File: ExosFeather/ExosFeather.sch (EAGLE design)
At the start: 3 parts, among them J1 CONN_3X1_JST_PA

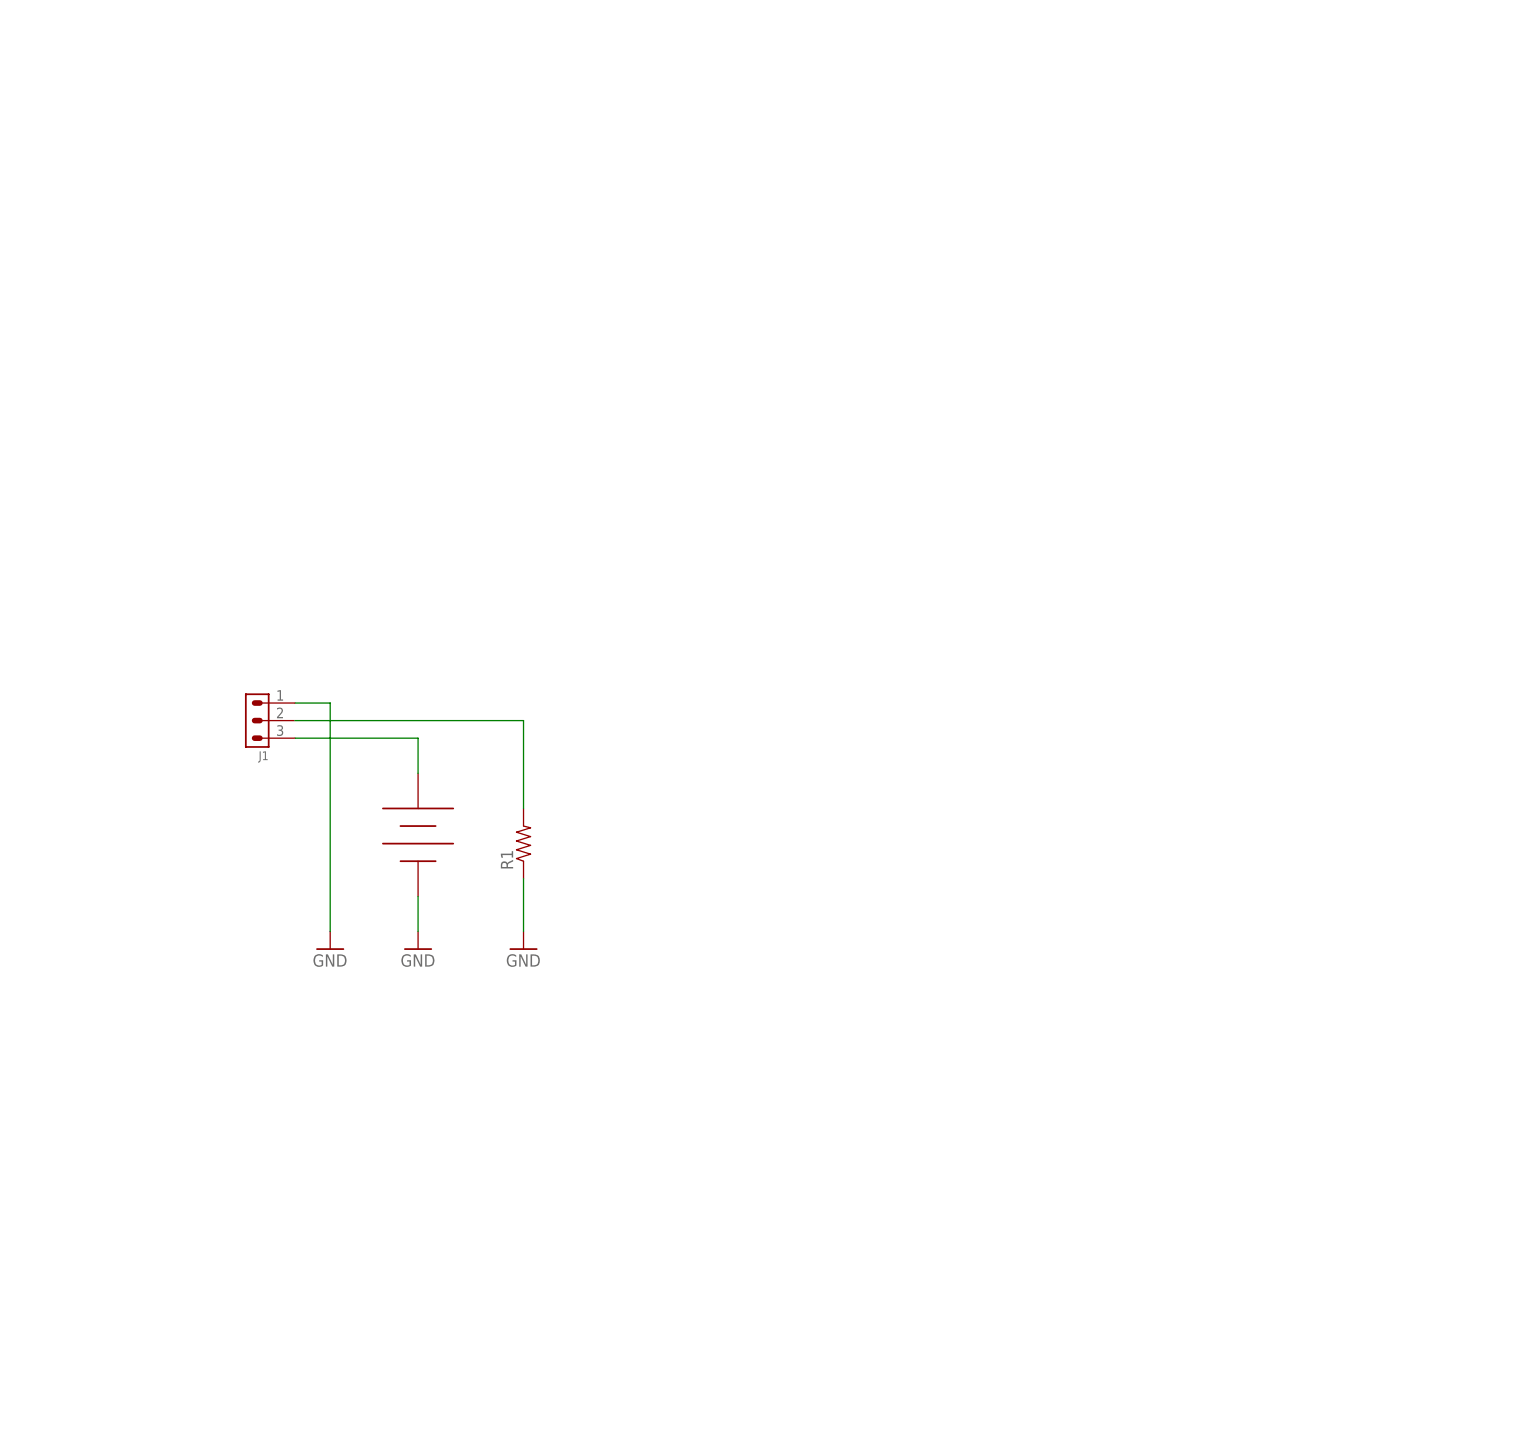
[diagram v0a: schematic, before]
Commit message: Revert "exosfeather"
This reverts commit d5dd059b457cfbbf08893ff69975569f2ea8e21c.
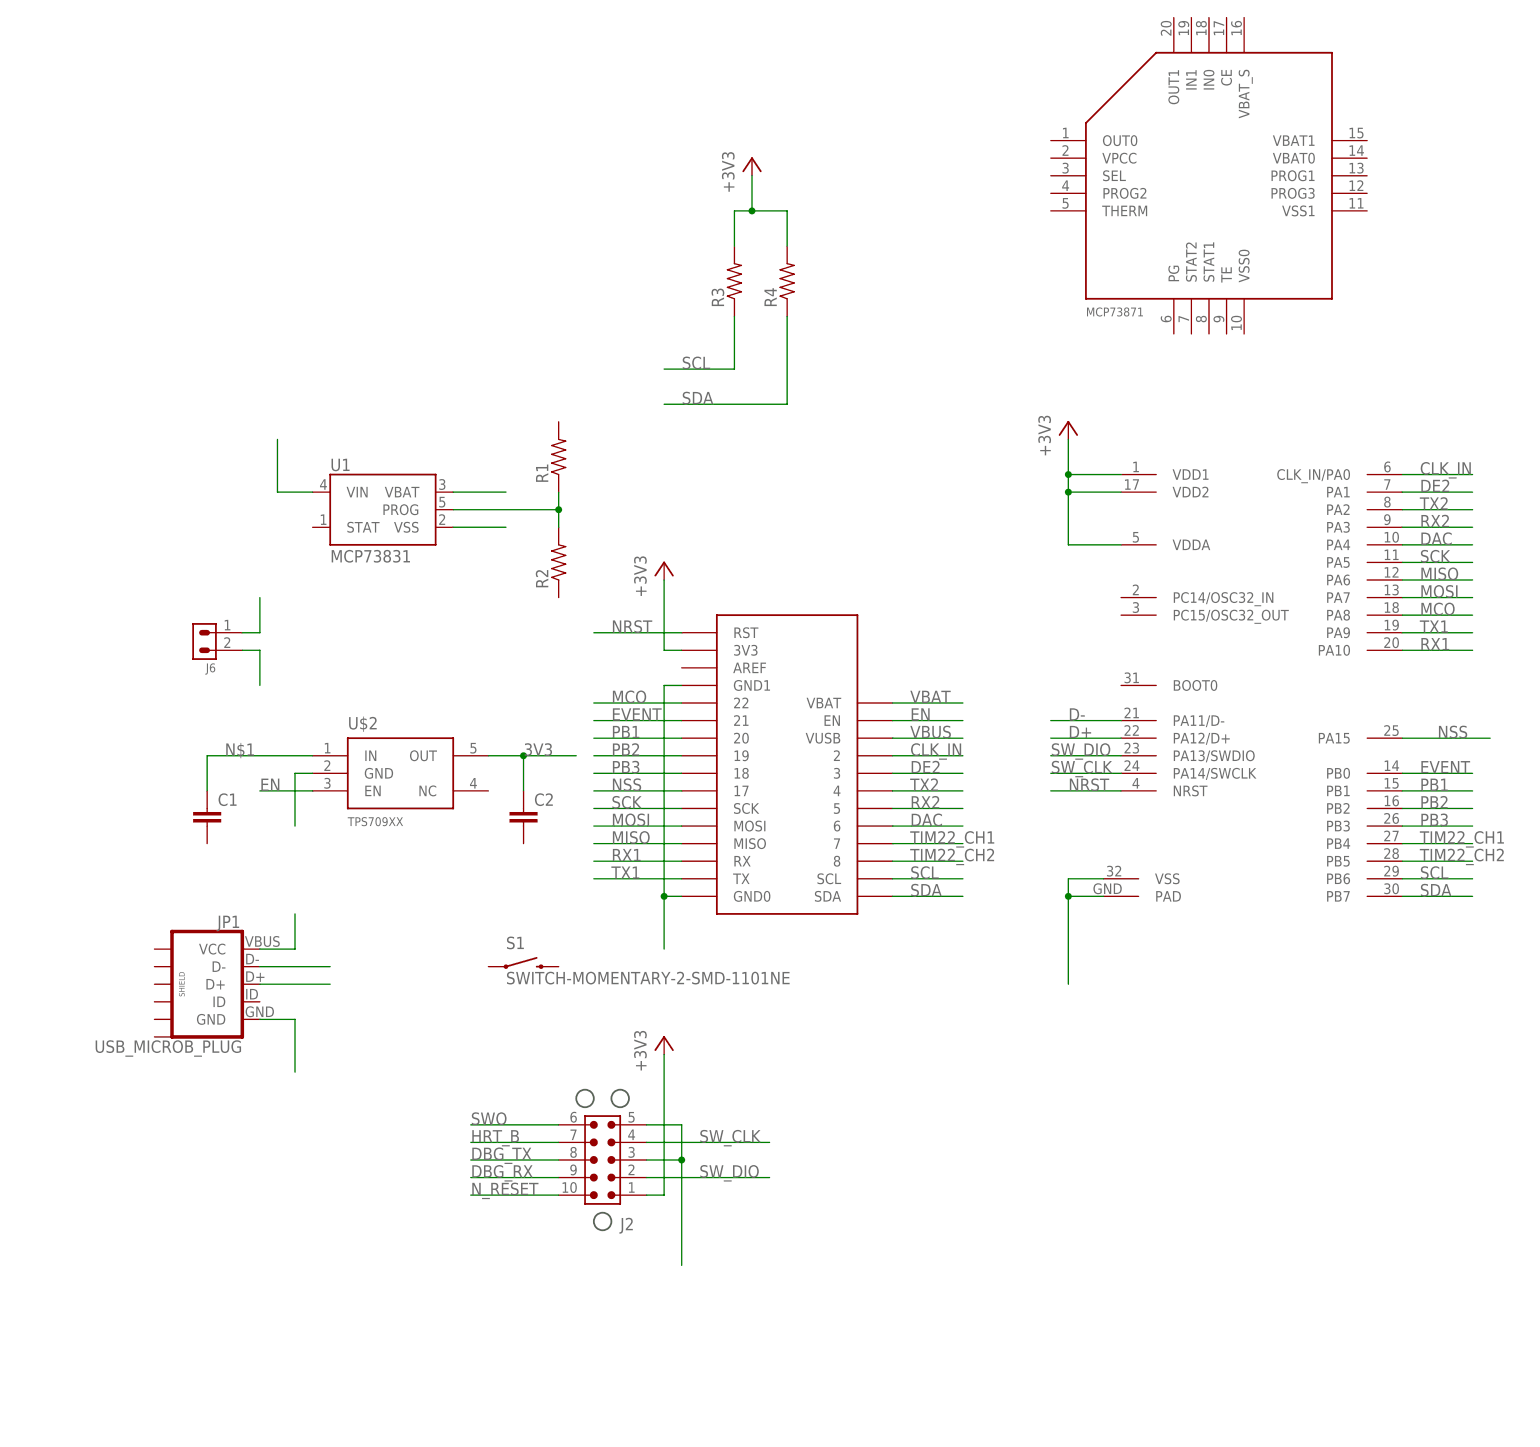
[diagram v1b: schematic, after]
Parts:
- removed J1: CONN_3X1_JST_PA, leaf:CONN_3X1_JST_PA
- added C1, C2: (no value), stepOSP:0603_CAP
- added J2: TC_2050_IDC_TOP, leaf:TC_2050_IDC_TOP
- added J6: CONN_2X1_JST_PA, leaf:CONN_2X1_JST_PA
- added JP1: USB_MICROB_PLUG, stepOSP:USB_MICROB_PLUG
- added R2, R3, R4: (no value), stepOSP:0603_RES
- added S1: SWITCH-MOMENTARY-2-SMD-1101NE, SparkFun-Electromechanical:SWITCH-MOMENTARY-2-SMD-1101NE
- added U$1: FEATHER_PINOUT_FULL, stepOSP:FEATHER_PINOUT_FULL
- added U$3: MCP73871, stepOSP:MCP73871
- added U1: MCP73831, SparkFun-PowerIC:MCP73831
- added U2: STM32L052KX, leaf:STM32L052KX
- U$2: value 14500_KEYSTONE_1024 -> TPS709XX; device stepOSP:14500_KEYSTONE_1024 -> stepOSP:TPS709XX
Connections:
- new net +3V3: J2.1, R3.2, R4.2, U$1.3V3, U2.VDD1, U2.VDD2, U2.VDDA
- new net 3V3: C2.1, U$2.OUT
- new net CLK_IN: U$1.2, U2.CLK_IN/PA0
- new net D+: JP1.D+, U2.PA12/D+
- new net D-: JP1.D-, U2.PA11/D-
- new net DAC: U$1.6, U2.PA4
- new net DBG_RX: J2.9
- new net DBG_TX: J2.8
- new net DE2: U$1.3, U2.PA1
- new net EN: U$1.EN, U$2.EN
- new net EVENT: U$1.21, U2.PB0
- new net HRT_B: J2.7
- new net MCO: U$1.22, U2.PA8
- new net MISO: U$1.MISO, U2.PA6
- new net MOSI: U$1.MOSI, U2.PA7
- new net N$3: U1.VIN
- new net N$4: J6.1
- new net N$5: R1.1, R2.2, U1.PROG
- new net N$6: U1.VBAT
- new net N$7: U1.VSS
- new net NRST: U$1.RST, U2.NRST
- new net NSS: U$1.17, U2.PA15
- new net N_RESET: J2.10
- new net PB1: U$1.20, U2.PB1
- new net PB2: U$1.19, U2.PB2
- new net PB3: U$1.18, U2.PB3
- new net RX1: U$1.RX, U2.PA10
- new net RX2: U$1.5, U2.PA3
- new net SCK: U$1.SCK, U2.PA5
- new net SCL: R3.1, U$1.SCL, U2.PB6
- new net SDA: R4.1, U$1.SDA, U2.PB7
- new net SWO: J2.6
- new net SW_CLK: J2.4, U2.PA14/SWCLK
- new net SW_DIO: J2.2, U2.PA13/SWDIO
- new net TIM22_CH1: U$1.7, U2.PB4
- new net TIM22_CH2: U$1.8, U2.PB5
- new net TX1: U$1.TX, U2.PA9
- new net TX2: U$1.4, U2.PA2
- new net VBAT: U$1.VBAT
- new net VBUS: U$1.VUSB
- net GND: now also J2.3, J2.5, J6.2, JP1.GND, U$1.GND0, U$1.GND1, U$2.GND, U2.PAD, U2.VSS; no longer J1.1, R1.1, U$2.NEG
- net N$1: now also C1.1, U$2.IN; no longer J1.2, R1.2
- net N$2: now also JP1.VCC; no longer J1.3, U$2.POS
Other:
- moved on the sheet: R1

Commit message: exofeather update
latest and greates exofeather
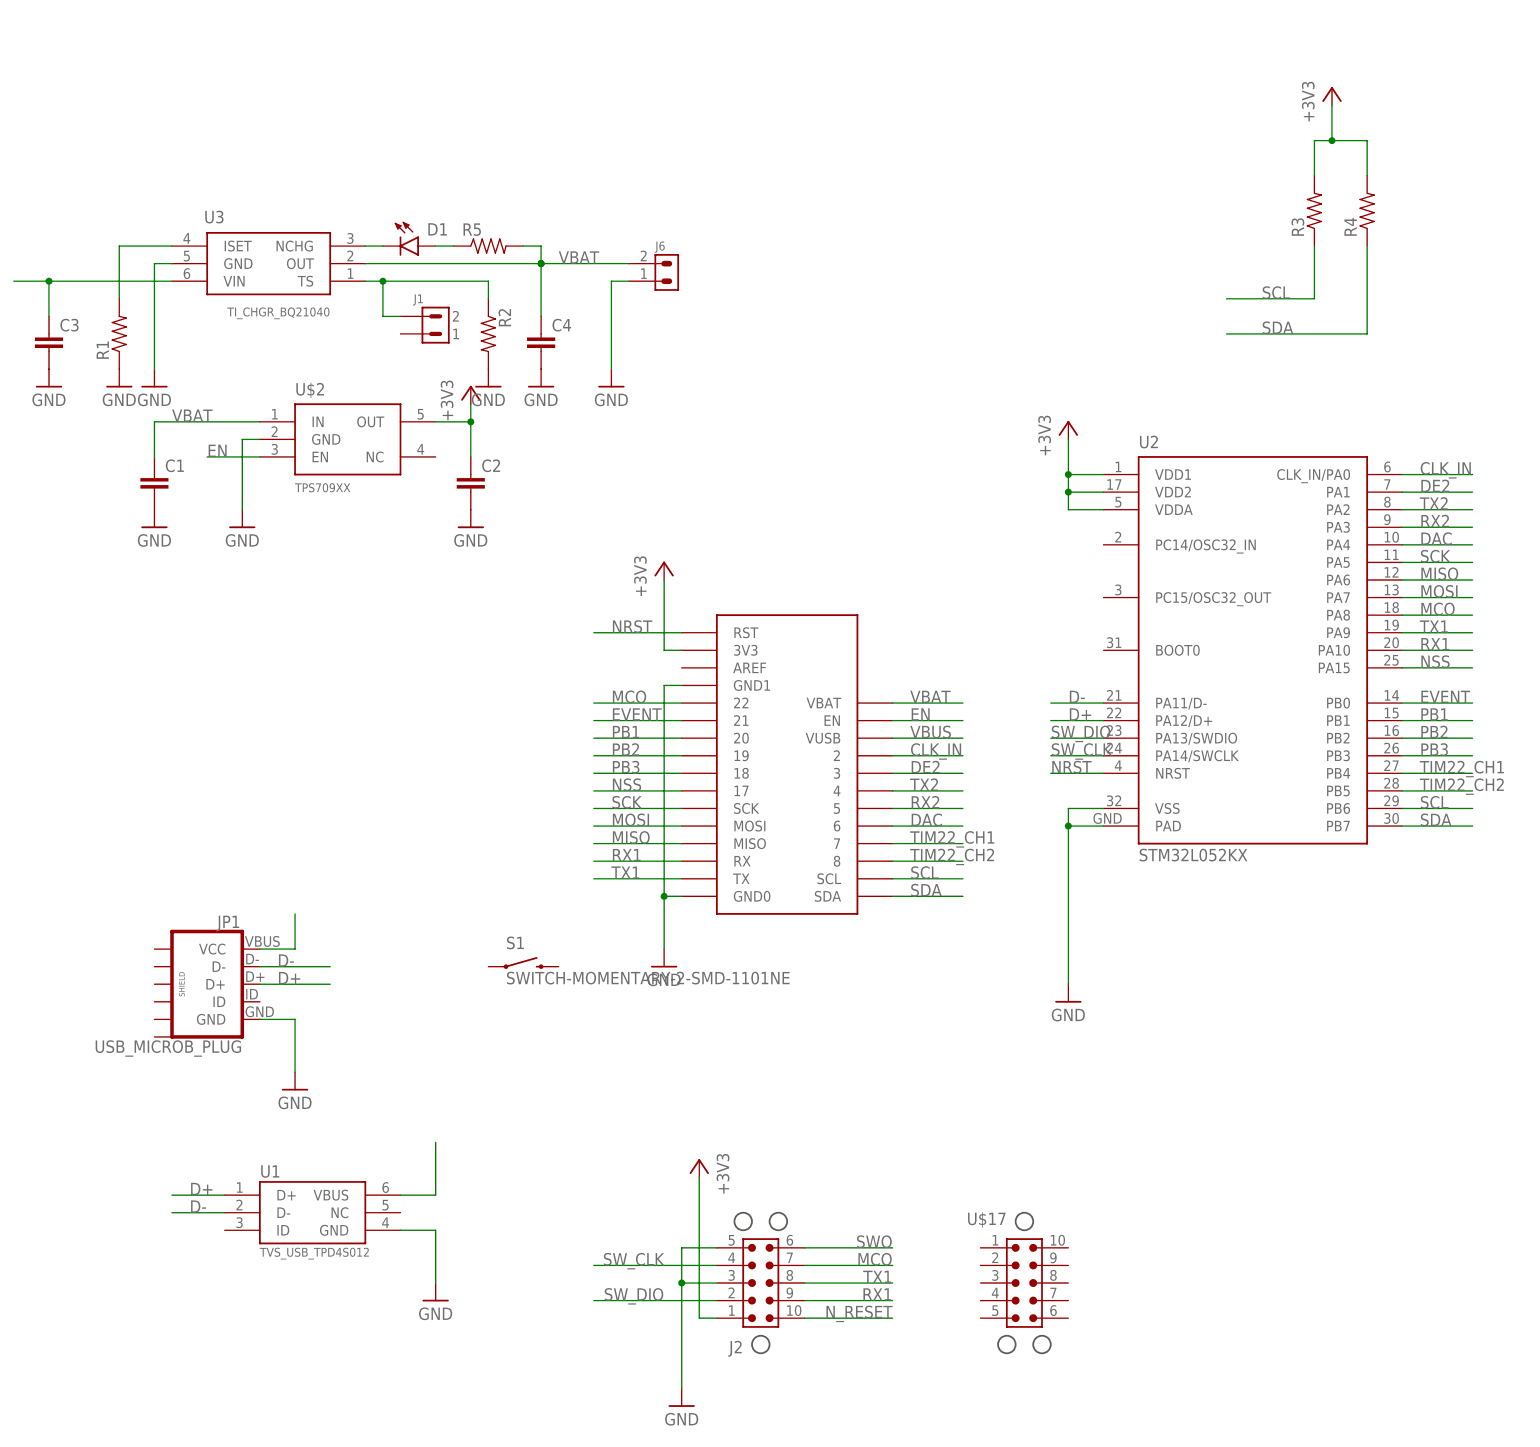
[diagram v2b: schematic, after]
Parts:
- removed U$3: MCP73871, stepOSP:MCP73871
- added C3, C4: (no value), stepOSP:0603_CAP
- added D1: 0603_LED, stepOSP:0603_LED
- added J1: JST_PH_2_PTH, stepOSP:JST_PH_2_PTH
- added R5: (no value), stepOSP:0603_RES
- added U$17: TC_2050_IDC_TOP, leaf:TC_2050_IDC_TOP
- added U3: TI_CHGR_BQ21040, leaf:TI_CHGR_BQ21040
- U1: value MCP73831 -> TVS_USB_TPD4S012; device SparkFun-PowerIC:MCP73831 -> leaf:TVS_USB_TPD4S012
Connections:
- removed net 3V3: C2.1, U$2.OUT
- removed net DBG_RX: J2.9
- removed net DBG_TX: J2.8
- removed net HRT_B: J2.7
- removed net N$1: C1.1, U$2.IN
- removed net N$2: JP1.VCC
- removed net N$4: J6.1
- net +3V3: now also C2.1, U$2.OUT
- net D+: now also U1.D+
- net D-: now also U1.D-
- net GND: now also C1.2, C2.2, C3.2, C4.2, J6.1, R1.1, R2.2, U1.GND, U3.GND; no longer J6.2
- net MCO: now also J2.7
- net N$3: now also J1.2, R2.1, U3.TS; no longer U1.VIN
- net N$5: now also R1.2, U3.ISET; no longer R1.1, R2.2, U1.PROG
- net N$6: now also D1.C, U3.NCHG; no longer U1.VBAT
- net N$7: now also D1.A, R5.1; no longer U1.VSS
- net RX1: now also J2.9
- net TX1: now also J2.8
- net VBAT: now also C1.1, C4.1, J6.2, R5.2, U$2.IN, U3.OUT
- net VBUS: now also C3.1, JP1.VCC, U1.VBUS, U3.VIN
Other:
- moved on the sheet: C1, C2, J2, J6, R1, R2, R3, R4, U$2
